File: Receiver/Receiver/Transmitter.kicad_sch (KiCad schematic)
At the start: 57 parts, among them J1 SSW-104-01-T-D-LL, J10 Conn_01x03, J11 Conn_01x03, J12 Conn_01x03, J13 Conn_01x03, J14 Conn_01x03, J2 105-1103-001, J3 Conn_01x06, J4 105-1103-001, J5 105-1103-001, J8 FCR7350R, J9 FCR7350R, Q1 RJF0408JPD-01#J3, Q10 RJF0408JPD-01#J3, Q3 RJF0408JPD-01#J3, Q5 RJF0408JPD-01#J3, Q6 RJF0408JPD-01#J3, Q9 RJF0408JPD-01#J3, SW1 D6R90F2LFS, SW2 500SSP1S2M2QEA, U1 ANT13SECQE, U2 STM32F030R8Tx, U3 MIC5205-3.3YM5, U4 TPS565201DDCR, U6 NRF24L01_Breakout, U7 HEF4104BT_653

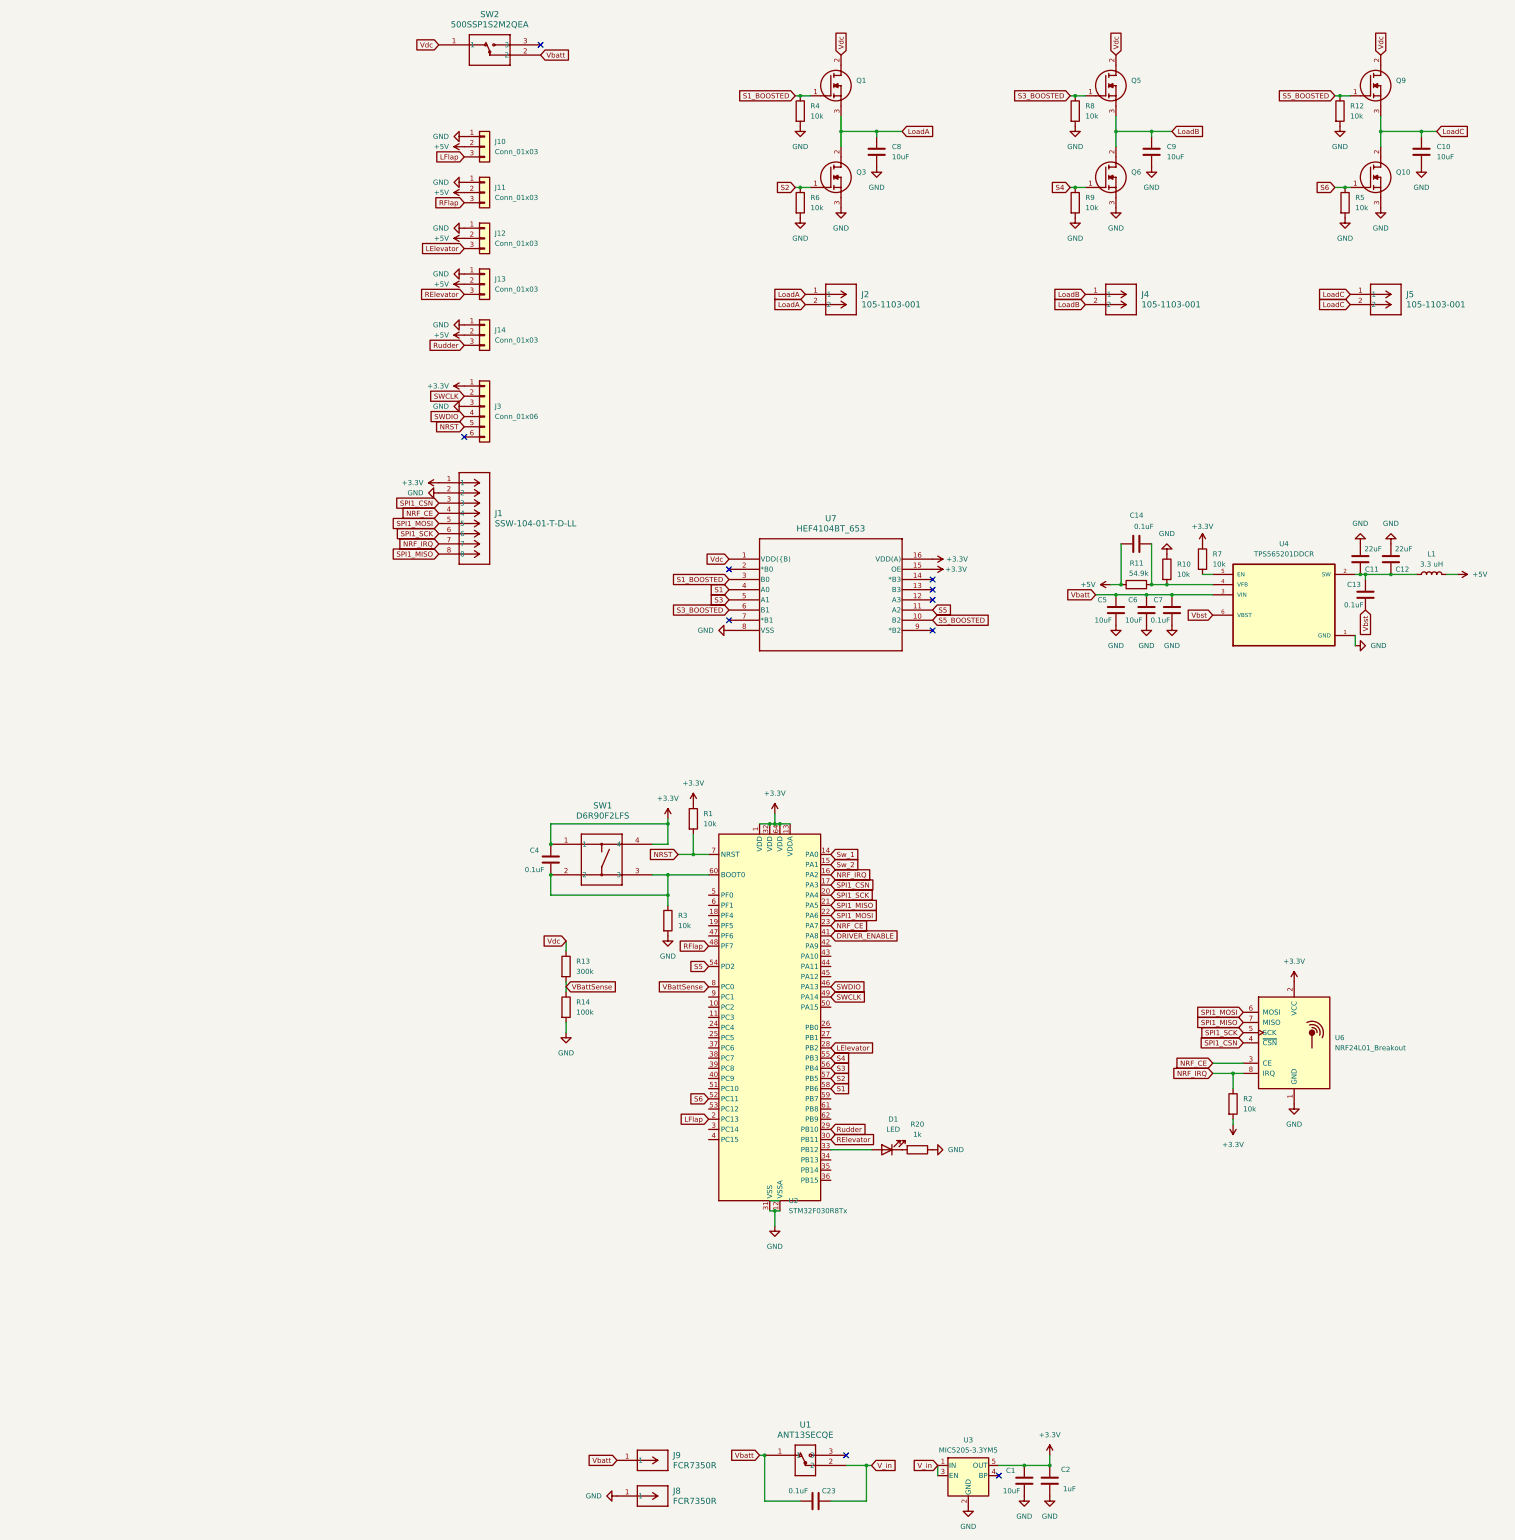
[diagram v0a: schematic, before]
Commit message: V2 PCB
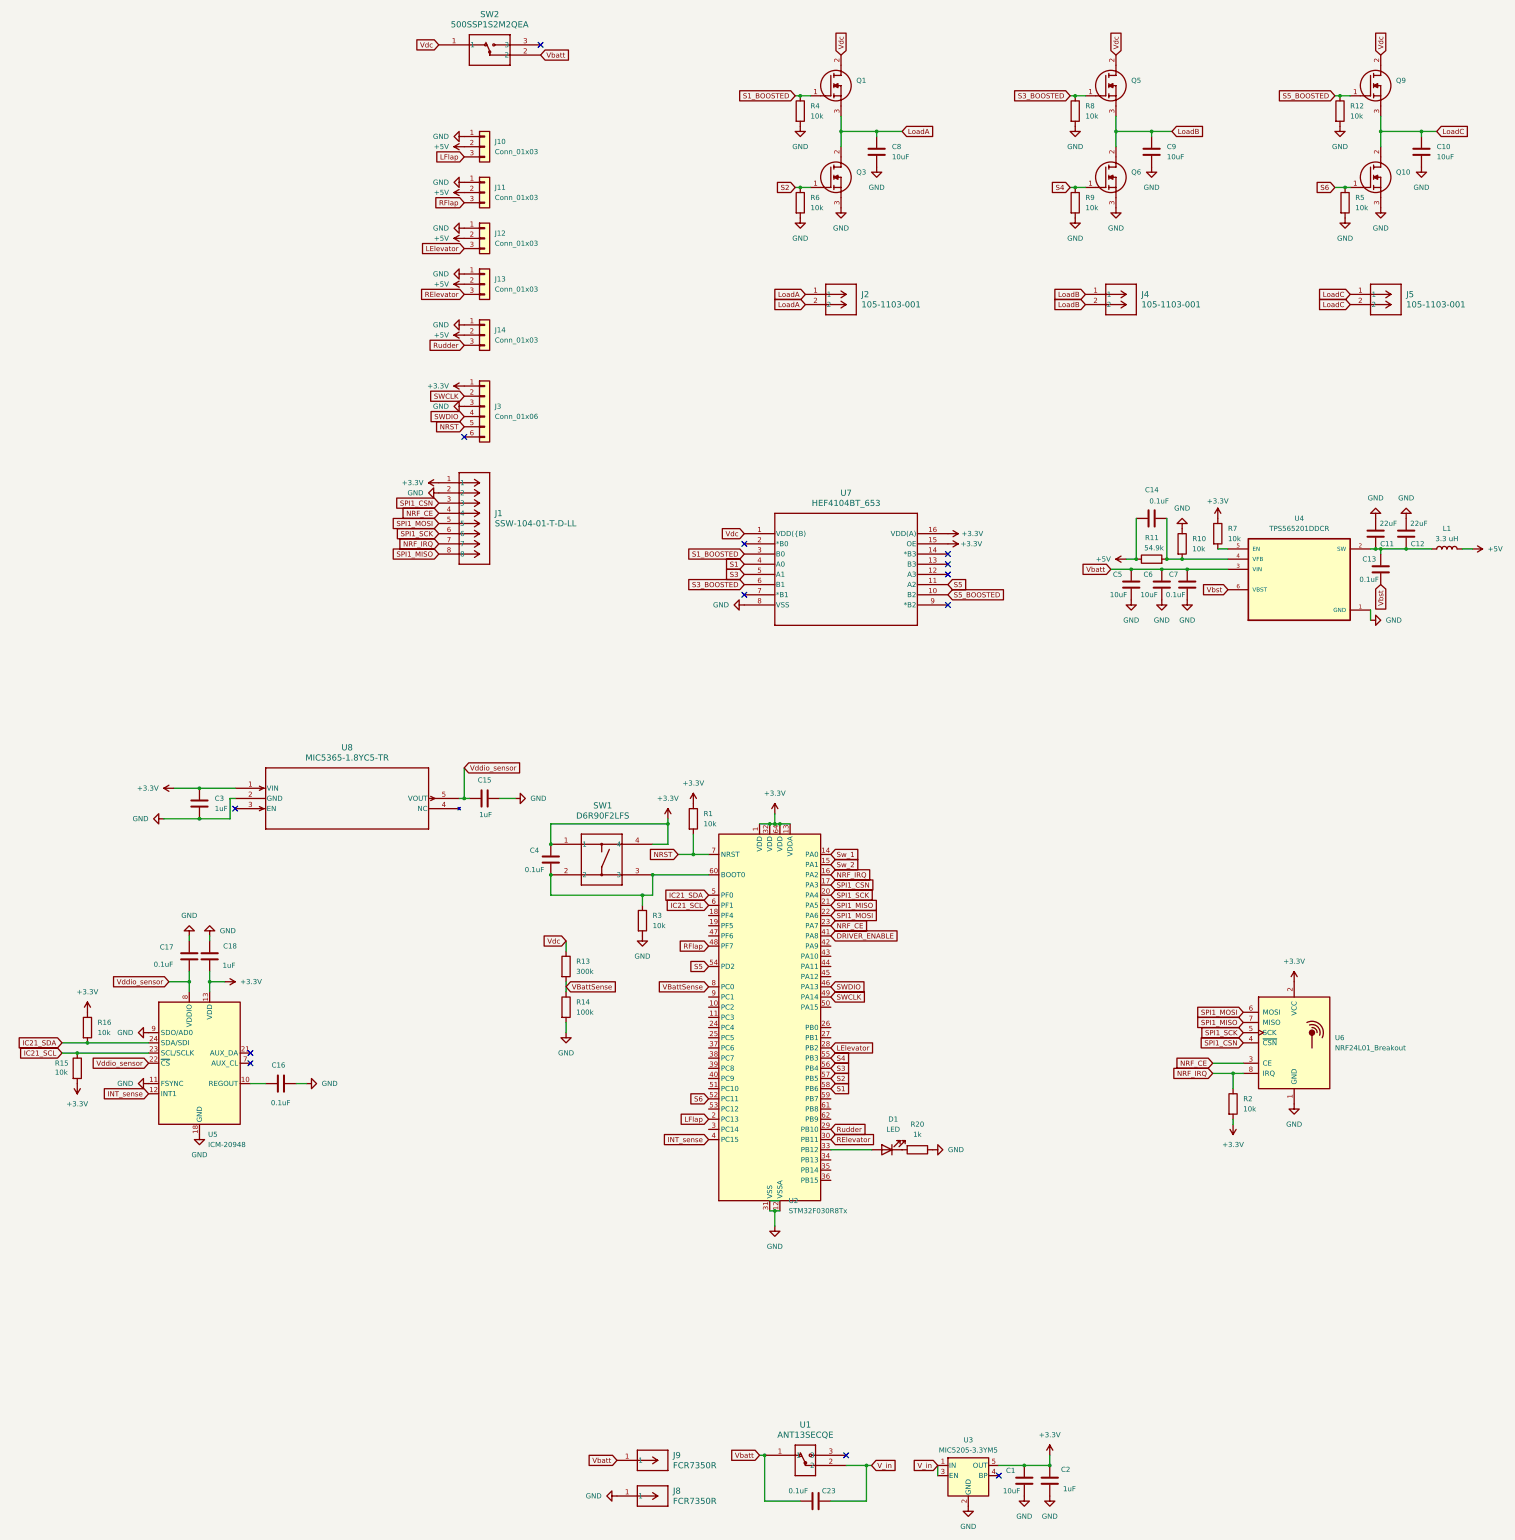
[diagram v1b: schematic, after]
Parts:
- added C15, C18, C3: 1uF, Capacitor_SMD:C_0402_1005Metric, symbol Device:C
- added C16, C17: 0.1uF, Capacitor_SMD:C_0402_1005Metric, symbol Device:C
- added R15, R16: 10k, Resistor_SMD:R_0402_1005Metric, symbol Device:R
- added U5: ICM-20948, Sensor_Motion:InvenSense_QFN-24_3x3mm_P0.4mm, symbol Sensor_Motion:ICM-20948
- added U8: MIC5365-1.8YC5-TR, Libary1:SC-70_C5_MCH, symbol MIC5365-1.8YC5-TR:MIC5365-1.8YC5-TR
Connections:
- net +3.3V: now also C18.1, C3.1, R15.2, R16.1, U5.13 (VDD), U8.1 (VIN)
- net GND: now also C15.2, C16.2, C17.1, C18.2, C3.2, U5.11 (FSYNC), U5.18 (GND), U5.20 (GND), U5.9 (SDO/AD0), U8.2 (GND)
- net INT_sense: now reaches U2.4 (PC15)
- net INT_sense: now also U5.12 (INT1)
- net IC21_SDA: now reaches U2.5 (PF0)
- net IC21_SDA: now also R16.2, U5.24 (SDA/SDI)
- net IC21_SCL: now reaches U2.6 (PF1)
- net IC21_SCL: now also R15.1, U5.23 (SCL/SCLK)
- new net: C16.1, U5.10 (REGOUT)
- new net Vddio_sensor: C15.1, C17.2, U5.22 (~{CS}), U5.8 (VDDIO), U8.5 (VOUT)
- no-connect marks 10 -> 13
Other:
- moved on the sheet: C11, C12, C13, C14, C5, C6, C7, L1, R10, R11, R3, R7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
